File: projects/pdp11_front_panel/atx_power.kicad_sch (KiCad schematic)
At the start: 1 part, among them J2 ATX-24

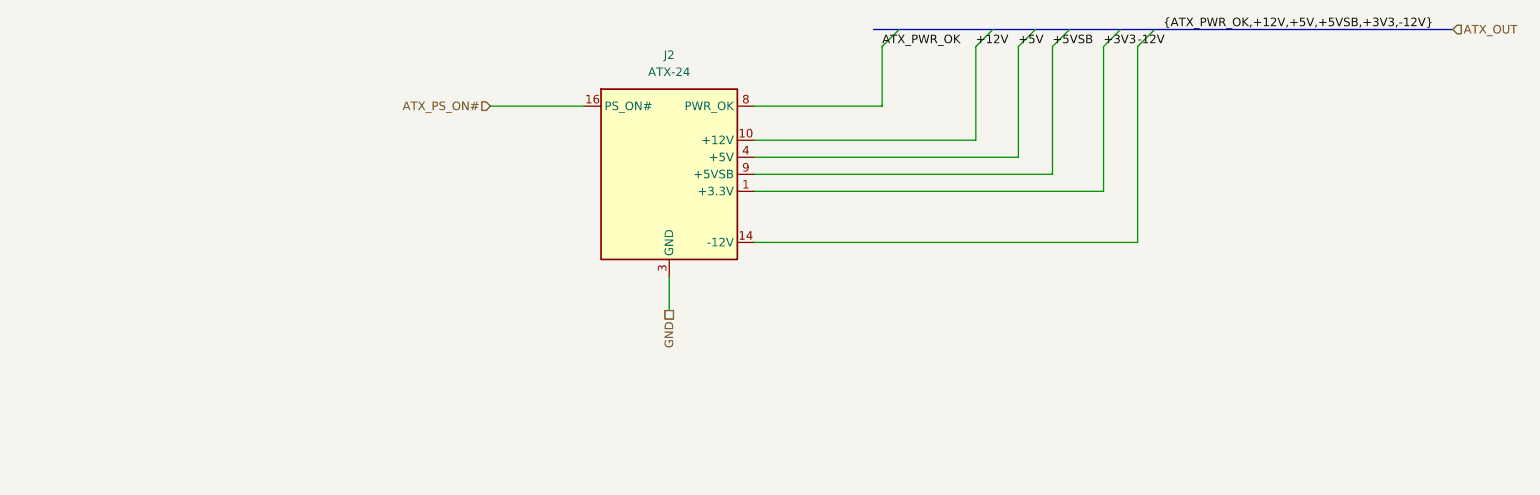
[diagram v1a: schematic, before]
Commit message: wip
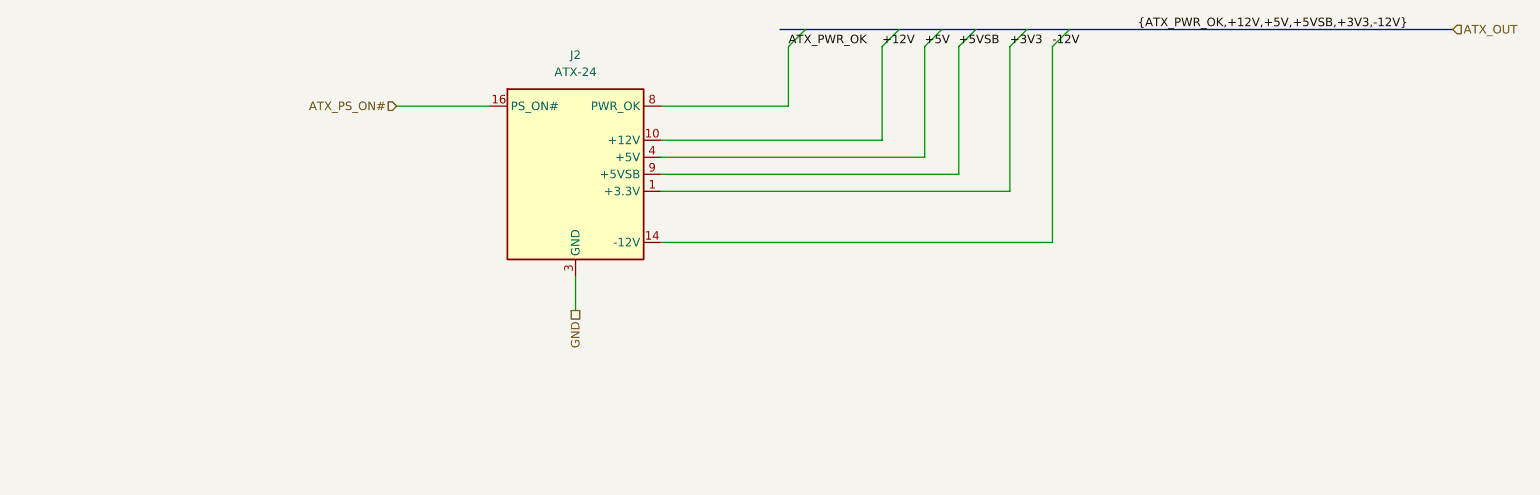
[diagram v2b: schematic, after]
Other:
- moved on the sheet: J2
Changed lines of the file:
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@@
 (kicad_sch (version 20230121) (generator eeschema)
   (paper "A4")
-  (bus_entry (at 196.85 55.88) (size -2.54 2.54)
+  (bus_entry (at 182.88 55.88) (size -2.54 2.54)
     (stroke (width 0) (type default))
   )
-  (bus_entry (at 190.5 55.88) (size -2.54 2.54)
+  (bus_entry (at 176.53 55.88) (size -2.54 2.54)
     (stroke (width 0) (type default))
   )
-  (bus_entry (at 209.55 55.88) (size -2.54 2.54)
+  (bus_entry (at 195.58 55.88) (size -2.54 2.54)
+    (stroke (width 0) (type default))
+  )
+  (bus_entry (at 187.96 55.88) (size -2.54 2.54)
     (stroke (width 0) (type default))
   )
@@
     (stroke (width 0) (type default))
   )
-  (bus_entry (at 214.63 55.88) (size -2.54 2.54)
+  (bus_entry (at 162.56 55.88) (size -2.54 2.54)
     (stroke (width 0) (type default))
   )
-  (bus_entry (at 176.53 55.88) (size -2.54 2.54)
+  (wire (pts (xy 140.97 77.47) (xy 185.42 77.47))
     (stroke (width 0) (type default))
   )
-  (wire (pts (xy 154.94 77.47) (xy 199.39 77.47))
+  (bus (pts (xy 182.88 55.88) (xy 187.96 55.88))
     (stroke (width 0) (type default))
   )
-  (bus (pts (xy 214.63 55.88) (xy 259.08 55.88))
+  (wire (pts (xy 140.97 74.93) (xy 180.34 74.93))
     (stroke (width 0) (type default))
   )
-  (bus (pts (xy 196.85 55.88) (xy 201.93 55.88))
+  (bus (pts (xy 162.56 55.88) (xy 176.53 55.88))
     (stroke (width 0) (type default))
   )
-  (wire (pts (xy 154.94 74.93) (xy 194.31 74.93))
+  (bus (pts (xy 187.96 55.88) (xy 195.58 55.88))
     (stroke (width 0) (type default))
   )
-  (bus (pts (xy 176.53 55.88) (xy 190.5 55.88))
+  (wire (pts (xy 140.97 80.01) (xy 193.04 80.01))
     (stroke (width 0) (type default))
   )
-  (bus (pts (xy 201.93 55.88) (xy 209.55 55.88))
+  (wire (pts (xy 160.02 58.42) (xy 160.02 67.31))
     (stroke (width 0) (type default))
   )
-  (wire (pts (xy 154.94 80.01) (xy 207.01 80.01))
+  (bus (pts (xy 201.93 55.88) (xy 259.08 55.88))
     (stroke (width 0) (type default))
   )
-  (wire (pts (xy 173.99 58.42) (xy 173.99 67.31))
+  (wire (pts (xy 101.6 67.31) (xy 115.57 67.31))
     (stroke (width 0) (type default))
   )
-  (wire (pts (xy 115.57 67.31) (xy 129.54 67.31))
+  (bus (pts (xy 176.53 55.88) (xy 182.88 55.88))
     (stroke (width 0) (type default))
   )
-  (bus (pts (xy 190.5 55.88) (xy 196.85 55.88))
+  (wire (pts (xy 193.04 80.01) (xy 193.04 58.42))
     (stroke (width 0) (type default))
   )
-  (wire (pts (xy 207.01 80.01) (xy 207.01 58.42))
+  (wire (pts (xy 160.02 67.31) (xy 140.97 67.31))
     (stroke (width 0) (type default))
   )
-  (wire (pts (xy 173.99 67.31) (xy 154.94 67.31))
+  (wire (pts (xy 199.39 58.42) (xy 199.39 87.63))
     (stroke (width 0) (type default))
   )
-  (wire (pts (xy 212.09 58.42) (xy 212.09 87.63))
+  (bus (pts (xy 158.75 55.88) (xy 162.56 55.88))
     (stroke (width 0) (type default))
   )
-  (bus (pts (xy 172.72 55.88) (xy 176.53 55.88))
+  (bus (pts (xy 195.58 55.88) (xy 201.93 55.88))
     (stroke (width 0) (type default))
   )
-  (bus (pts (xy 209.55 55.88) (xy 214.63 55.88))
+  (wire (pts (xy 180.34 58.42) (xy 180.34 74.93))
     (stroke (width 0) (type default))
   )
-  (wire (pts (xy 194.31 58.42) (xy 194.31 74.93))
+  (wire (pts (xy 185.42 77.47) (xy 185.42 58.42))
     (stroke (width 0) (type default))
   )
-  (wire (pts (xy 199.39 77.47) (xy 199.39 58.42))
+  (wire (pts (xy 128.27 92.71) (xy 128.27 97.79))
     (stroke (width 0) (type default))
   )
-  (wire (pts (xy 142.24 92.71) (xy 142.24 97.79))
+  (wire (pts (xy 140.97 87.63) (xy 199.39 87.63))
     (stroke (width 0) (type default))
   )
-  (wire (pts (xy 154.94 87.63) (xy 212.09 87.63))
+  (wire (pts (xy 140.97 72.39) (xy 173.99 72.39))
     (stroke (width 0) (type default))
   )
-  (wire (pts (xy 154.94 72.39) (xy 187.96 72.39))
+  (wire (pts (xy 173.99 58.42) (xy 173.99 72.39))
     (stroke (width 0) (type default))
   )
-  (wire (pts (xy 187.96 58.42) (xy 187.96 72.39))
-    (stroke (width 0) (type default))
-  )
-  (label "{ATX_PWR_OK,+12V,+5V,+5VSB,+3V3,-12V}" (at 215.9 55.88 0) (fields_autoplaced)
+  (label "{ATX_PWR_OK,+12V,+5V,+5VSB,+3V3,-12V}" (at 212.09 55.88 0) (fields_autoplaced)
     (effects (font (size 1.27 1.27)) (justify left bottom))
   )
-  (label "-12V" (at 212.09 58.42 0) (fields_autoplaced)
+  (label "-12V" (at 199.39 58.42 0) (fields_autoplaced)
     (effects (font (size 1.27 1.27)) (justify left bottom))
   )
-  (label "+12V" (at 187.96 58.42 0) (fields_autoplaced)
+  (label "+12V" (at 173.99 58.42 0) (fields_autoplaced)
     (effects (font (size 1.27 1.27)) (justify left bottom))
   )
-  (label "ATX_PWR_OK" (at 173.99 58.42 0) (fields_autoplaced)
+  (label "ATX_PWR_OK" (at 160.02 58.42 0) (fields_autoplaced)
     (effects (font (size 1.27 1.27)) (justify left bottom))
   )
-  (label "+5V" (at 194.31 58.42 0) (fields_autoplaced)
+  (label "+5V" (at 180.34 58.42 0) (fields_autoplaced)
     (effects (font (size 1.27 1.27)) (justify left bottom))
   )
-  (label "+3V3" (at 207.01 58.42 0) (fields_autoplaced)
+  (label "+3V3" (at 193.04 58.42 0) (fields_autoplaced)
     (effects (font (size 1.27 1.27)) (justify left bottom))
   )
-  (label "+5VSB" (at 199.39 58.42 0) (fields_autoplaced)
+  (label "+5VSB" (at 185.42 58.42 0) (fields_autoplaced)
     (effects (font (size 1.27 1.27)) (justify left bottom))
   )
@@
     (effects (font (size 1.27 1.27)) (justify left))
   )
-  (hierarchical_label "GND" (shape passive) (at 142.24 97.79 270) (fields_autoplaced)
+  (hierarchical_label "GND" (shape passive) (at 128.27 97.79 270) (fields_autoplaced)
     (effects (font (size 1.27 1.27)) (justify right))
   )
-  (hierarchical_label "ATX_PS_ON#" (shape input) (at 115.57 67.31 180) (fields_autoplaced)
+  (hierarchical_label "ATX_PS_ON#" (shape input) (at 101.6 67.31 180) (fields_autoplaced)
     (effects (font (size 1.27 1.27)) (justify right))
   )
-  (symbol (lib_id "Connector:ATX-24") (at 142.24 77.47 0) (unit 1)
+  (symbol (lib_id "Connector:ATX-24") (at 128.27 77.47 0) (unit 1)
     (in_bom yes) (on_board yes) (dnp no) (fields_autoplaced)
-    (property "Reference" "J2" (at 142.24 59.69 0)
+    (property "Reference" "J2" (at 128.27 59.69 0)
       (effects (font (size 1.27 1.27)))
     )
-    (property "Value" "ATX-24" (at 142.24 62.23 0)
+    (property "Value" "ATX-24" (at 128.27 62.23 0)
       (effects (font (size 1.27 1.27)))
     )
-    (property "Footprint" "" (at 142.24 80.01 0)
+    (property "Footprint" "" (at 128.27 80.01 0)
       (effects (font (size 1.27 1.27)) hide)
     )
-    (property "Datasheet" "https://www.intel.com/content/dam/www/public/us/en/documents/guides/power-supply-design-guide-june.pdf#page=33" (at 203.2 91.44 0)
+    (property "Datasheet" "https://www.intel.com/content/dam/www/public/us/en/documents/guides/power-supply-design-guide-june.pdf#page=33" (at 189.23 91.44 0)
       (effects (font (size 1.27 1.27)) hide)
     )

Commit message: wip
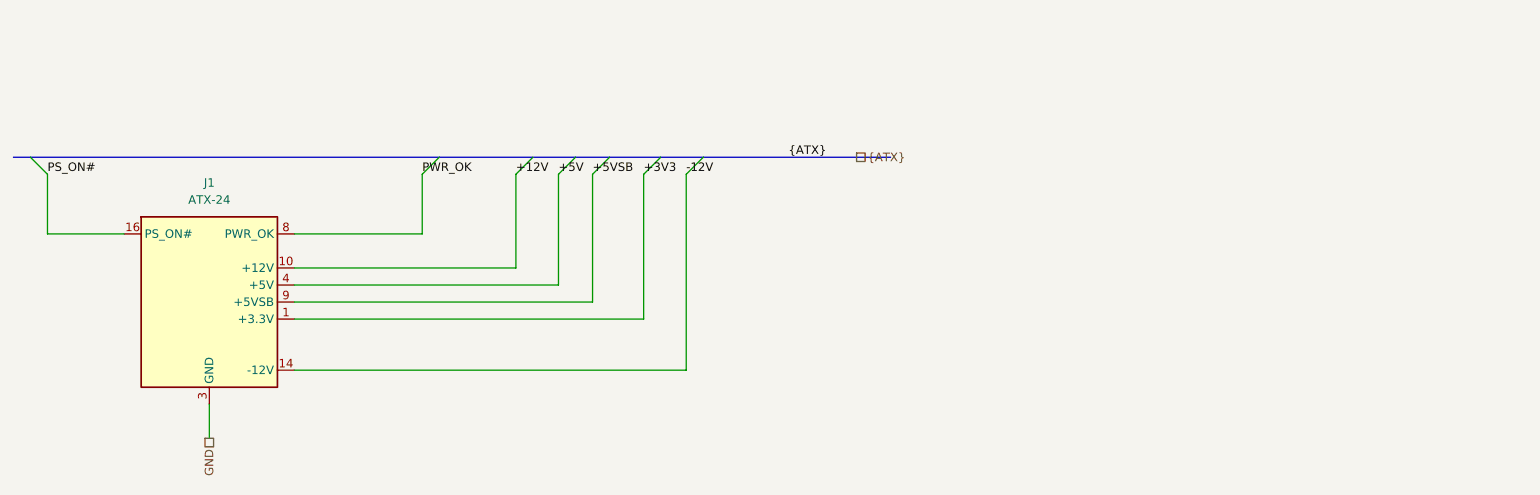
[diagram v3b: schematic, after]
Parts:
- renumbered J2 to J1
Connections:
- net ATX_PS_ON# renamed PS_ON#
- net ATX_PWR_OK renamed PWR_OK
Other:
- moved on the sheet: J1
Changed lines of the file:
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@@
 (kicad_sch (version 20230121) (generator eeschema)
   (paper "A4")
-  (bus_entry (at 182.88 55.88) (size -2.54 2.54)
+  (bus_entry (at 128.27 74.93) (size -2.54 2.54)
     (stroke (width 0) (type default))
   )
-  (bus_entry (at 176.53 55.88) (size -2.54 2.54)
+  (bus_entry (at 121.92 74.93) (size -2.54 2.54)
     (stroke (width 0) (type default))
   )
-  (bus_entry (at 195.58 55.88) (size -2.54 2.54)
+  (bus_entry (at 140.97 74.93) (size -2.54 2.54)
     (stroke (width 0) (type default))
   )
-  (bus_entry (at 187.96 55.88) (size -2.54 2.54)
+  (bus_entry (at 133.35 74.93) (size -2.54 2.54)
     (stroke (width 0) (type default))
   )
-  (bus_entry (at 201.93 55.88) (size -2.54 2.54)
+  (bus_entry (at 46.99 74.93) (size 2.54 2.54)
     (stroke (width 0) (type default))
   )
-  (bus_entry (at 162.56 55.88) (size -2.54 2.54)
+  (bus_entry (at 147.32 74.93) (size -2.54 2.54)
     (stroke (width 0) (type default))
   )
-  (wire (pts (xy 140.97 77.47) (xy 185.42 77.47))
+  (bus_entry (at 107.95 74.93) (size -2.54 2.54)
     (stroke (width 0) (type default))
   )
-  (bus (pts (xy 182.88 55.88) (xy 187.96 55.88))
+  (wire (pts (xy 86.36 96.52) (xy 130.81 96.52))
     (stroke (width 0) (type default))
   )
-  (wire (pts (xy 140.97 74.93) (xy 180.34 74.93))
+  (wire (pts (xy 86.36 93.98) (xy 125.73 93.98))
     (stroke (width 0) (type default))
   )
-  (bus (pts (xy 162.56 55.88) (xy 176.53 55.88))
+  (bus (pts (xy 107.95 74.93) (xy 121.92 74.93))
     (stroke (width 0) (type default))
   )
-  (bus (pts (xy 187.96 55.88) (xy 195.58 55.88))
+  (wire (pts (xy 86.36 99.06) (xy 138.43 99.06))
     (stroke (width 0) (type default))
   )
-  (wire (pts (xy 140.97 80.01) (xy 193.04 80.01))
+  (wire (pts (xy 105.41 77.47) (xy 105.41 86.36))
     (stroke (width 0) (type default))
   )
-  (wire (pts (xy 160.02 58.42) (xy 160.02 67.31))
+  (wire (pts (xy 49.53 77.47) (xy 49.53 86.36))
     (stroke (width 0) (type default))
   )
-  (bus (pts (xy 201.93 55.88) (xy 259.08 55.88))
+  (bus (pts (xy 128.27 74.93) (xy 133.35 74.93))
     (stroke (width 0) (type default))
   )
-  (wire (pts (xy 101.6 67.31) (xy 115.57 67.31))
+  (bus (pts (xy 121.92 74.93) (xy 128.27 74.93))
     (stroke (width 0) (type default))
   )
-  (bus (pts (xy 176.53 55.88) (xy 182.88 55.88))
+  (bus (pts (xy 140.97 74.93) (xy 147.32 74.93))
     (stroke (width 0) (type default))
   )
-  (wire (pts (xy 193.04 80.01) (xy 193.04 58.42))
+  (wire (pts (xy 138.43 99.06) (xy 138.43 77.47))
     (stroke (width 0) (type default))
   )
-  (wire (pts (xy 160.02 67.31) (xy 140.97 67.31))
+  (bus (pts (xy 147.32 74.93) (xy 175.26 74.93))
     (stroke (width 0) (type default))
   )
-  (wire (pts (xy 199.39 58.42) (xy 199.39 87.63))
+  (wire (pts (xy 105.41 86.36) (xy 86.36 86.36))
     (stroke (width 0) (type default))
   )
-  (bus (pts (xy 158.75 55.88) (xy 162.56 55.88))
+  (bus (pts (xy 44.45 74.93) (xy 46.99 74.93))
     (stroke (width 0) (type default))
   )
-  (bus (pts (xy 195.58 55.88) (xy 201.93 55.88))
+  (wire (pts (xy 144.78 77.47) (xy 144.78 106.68))
     (stroke (width 0) (type default))
   )
-  (wire (pts (xy 180.34 58.42) (xy 180.34 74.93))
+  (bus (pts (xy 133.35 74.93) (xy 140.97 74.93))
     (stroke (width 0) (type default))
   )
-  (wire (pts (xy 185.42 77.47) (xy 185.42 58.42))
+  (wire (pts (xy 49.53 86.36) (xy 60.96 86.36))
     (stroke (width 0) (type default))
   )
-  (wire (pts (xy 128.27 92.71) (xy 128.27 97.79))
+  (wire (pts (xy 125.73 77.47) (xy 125.73 93.98))
     (stroke (width 0) (type default))
   )
-  (wire (pts (xy 140.97 87.63) (xy 199.39 87.63))
+  (wire (pts (xy 130.81 96.52) (xy 130.81 77.47))
     (stroke (width 0) (type default))
   )
-  (wire (pts (xy 140.97 72.39) (xy 173.99 72.39))
+  (bus (pts (xy 46.99 74.93) (xy 107.95 74.93))
     (stroke (width 0) (type default))
   )
-  (wire (pts (xy 173.99 58.42) (xy 173.99 72.39))
+  (wire (pts (xy 73.66 111.76) (xy 73.66 116.84))
     (stroke (width 0) (type default))
   )
-  (label "{ATX_PWR_OK,+12V,+5V,+5VSB,+3V3,-12V}" (at 212.09 55.88 0) (fields_autoplaced)
+  (wire (pts (xy 86.36 106.68) (xy 144.78 106.68))
+    (stroke (width 0) (type default))
+  )
+  (wire (pts (xy 86.36 91.44) (xy 119.38 91.44))
+    (stroke (width 0) (type default))
+  )
+  (wire (pts (xy 119.38 77.47) (xy 119.38 91.44))
+    (stroke (width 0) (type default))
+  )
+  (label "PS_ON#" (at 49.53 77.47 0) (fields_autoplaced)
     (effects (font (size 1.27 1.27)) (justify left bottom))
   )
-  (label "-12V" (at 199.39 58.42 0) (fields_autoplaced)
+  (label "-12V" (at 144.78 77.47 0) (fields_autoplaced)
     (effects (font (size 1.27 1.27)) (justify left bottom))
   )
-  (label "+12V" (at 173.99 58.42 0) (fields_autoplaced)
+  (label "+12V" (at 119.38 77.47 0) (fields_autoplaced)
     (effects (font (size 1.27 1.27)) (justify left bottom))
   )
-  (label "ATX_PWR_OK" (at 160.02 58.42 0) (fields_autoplaced)
+  (label "PWR_OK" (at 105.41 77.47 0) (fields_autoplaced)
     (effects (font (size 1.27 1.27)) (justify left bottom))
   )
-  (label "+5V" (at 180.34 58.42 0) (fields_autoplaced)
+  (label "+5V" (at 125.73 77.47 0) (fields_autoplaced)
     (effects (font (size 1.27 1.27)) (justify left bottom))
   )
-  (label "+3V3" (at 193.04 58.42 0) (fields_autoplaced)
+  (label "+3V3" (at 138.43 77.47 0) (fields_autoplaced)
     (effects (font (size 1.27 1.27)) (justify left bottom))
   )
-  (label "+5VSB" (at 185.42 58.42 0) (fields_autoplaced)
+  (label "{ATX}" (at 160.02 74.93 0) (fields_autoplaced)
     (effects (font (size 1.27 1.27)) (justify left bottom))
   )
-  (hierarchical_label "ATX_OUT" (shape input) (at 259.08 55.88 0) (fields_autoplaced)
+  (label "+5VSB" (at 130.81 77.47 0) (fields_autoplaced)
+    (effects (font (size 1.27 1.27)) (justify left bottom))
+  )
+  (hierarchical_label "{ATX}" (shape passive) (at 170.18 74.93 0) (fields_autoplaced)
     (effects (font (size 1.27 1.27)) (justify left))
   )
-  (hierarchical_label "GND" (shape passive) (at 128.27 97.79 270) (fields_autoplaced)
+  (hierarchical_label "GND" (shape passive) (at 73.66 116.84 270) (fields_autoplaced)
     (effects (font (size 1.27 1.27)) (justify right))
   )
-  (hierarchical_label "ATX_PS_ON#" (shape input) (at 101.6 67.31 180) (fields_autoplaced)
-    (effects (font (size 1.27 1.27)) (justify right))
-  )
-  (symbol (lib_id "Connector:ATX-24") (at 128.27 77.47 0) (unit 1)
+  (symbol (lib_id "Connector:ATX-24") (at 73.66 96.52 0) (unit 1)
     (in_bom yes) (on_board yes) (dnp no) (fields_autoplaced)
-    (property "Reference" "J2" (at 128.27 59.69 0)
+    (property "Reference" "J1" (at 73.66 78.74 0)
       (effects (font (size 1.27 1.27)))
     )
-    (property "Value" "ATX-24" (at 128.27 62.23 0)
+    (property "Value" "ATX-24" (at 73.66 81.28 0)
       (effects (font (size 1.27 1.27)))
     )
-    (property "Footprint" "" (at 128.27 80.01 0)
+    (property "Footprint" "" (at 73.66 99.06 0)
       (effects (font (size 1.27 1.27)) hide)
     )
-    (property "Datasheet" "https://www.intel.com/content/dam/www/public/us/en/documents/guides/power-supply-design-guide-june.pdf#page=33" (at 189.23 91.44 0)
+    (property "Datasheet" "https://www.intel.com/content/dam/www/public/us/en/documents/guides/power-supply-design-guide-june.pdf#page=33" (at 134.62 110.49 0)
       (effects (font (size 1.27 1.27)) hide)
     )
@@
       (project "pdp11_front_panel"
         (path "/e63e39d7-6ac0-4ffd-8aa3-1841a4541b55/d4d8f7cc-faea-4935-ab3d-bc61af3c0a31"
-          (reference "J2") (unit 1)
+          (reference "J1") (unit 1)
         )
       )

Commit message: wip
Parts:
- J1: footprint (none) -> Connector_Molex:Molex_Mini-Fit_Jr_5569-24A1_2x12_P4.20mm_Horizontal
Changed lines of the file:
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@@
       (effects (font (size 1.27 1.27)))
     )
-    (property "Footprint" "" (at 73.66 99.06 0)
+    (property "Footprint" "Connector_Molex:Molex_Mini-Fit_Jr_5569-24A1_2x12_P4.20mm_Horizontal" (at 73.66 99.06 0)
       (effects (font (size 1.27 1.27)) hide)
     )
